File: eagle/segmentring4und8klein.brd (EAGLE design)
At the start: 100 x 150 mm, 12 parts

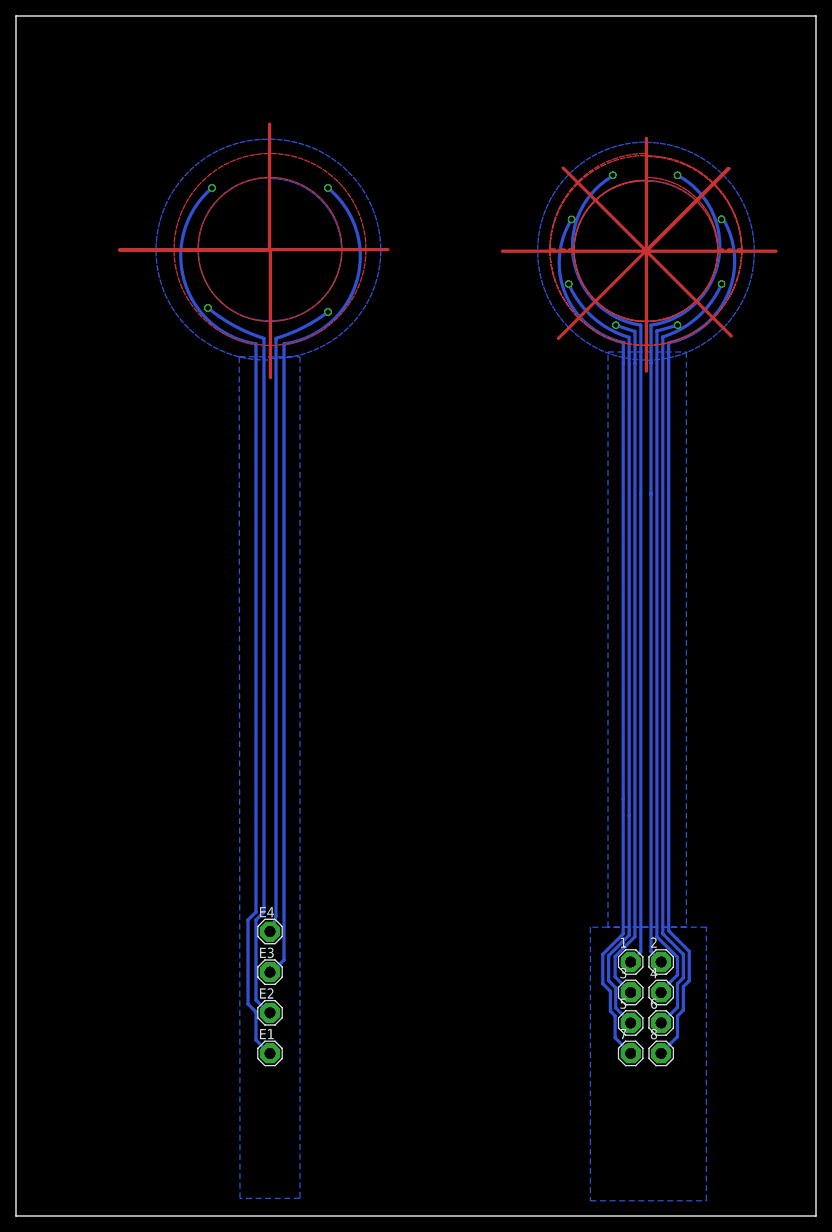
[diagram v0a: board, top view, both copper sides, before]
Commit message: Verbesserung der Boards
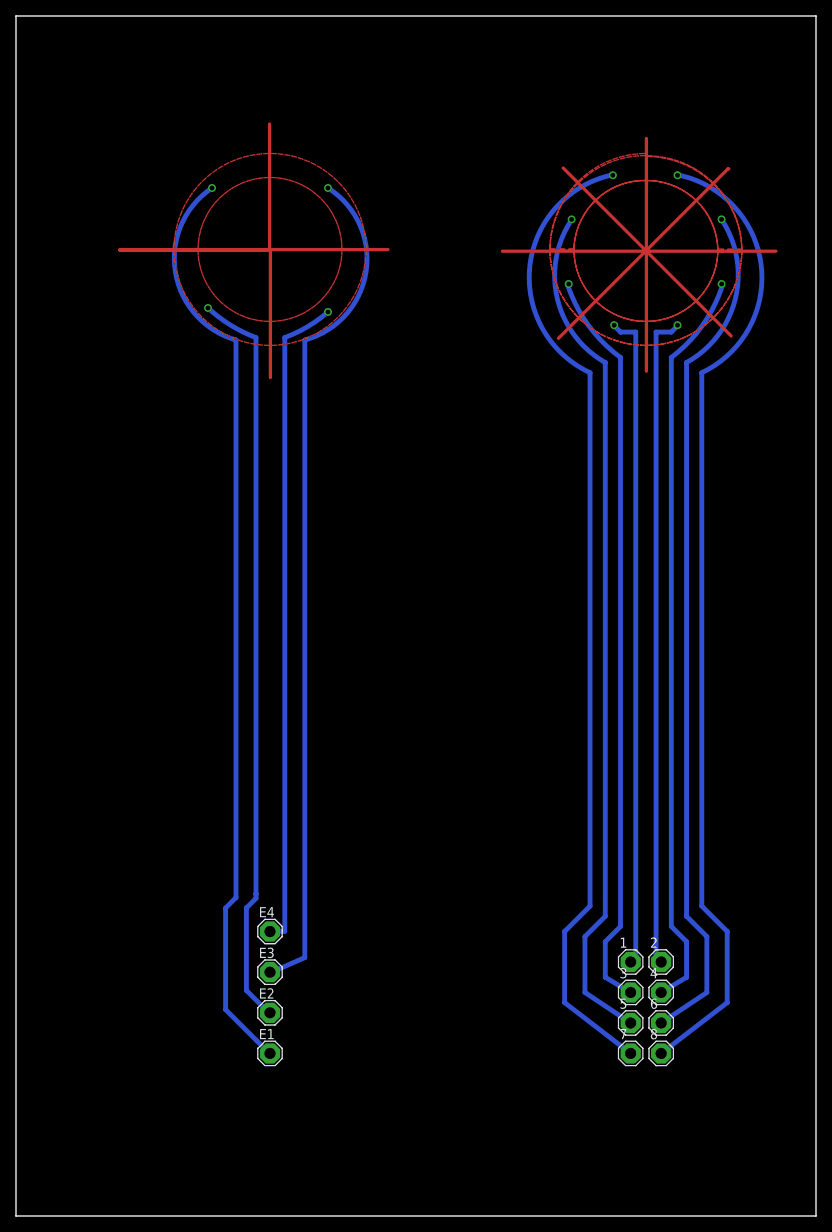
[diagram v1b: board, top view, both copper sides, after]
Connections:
- new net 1: 1.MP
- new net 2: 2.MP
- new net 3: 3.MP
- new net 4: 4.MP
- new net 5: 5.MP
- new net 6: 6.MP
- new net 7: 7.MP
- new net 8: 8.MP
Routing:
- net S$3: track 137.6 -> 93.0 mm
- net S$4: track 0.00 -> 30.1 mm
- net 2: track 99.7 -> 81.8 mm
- net 1: track 99.1 -> 81.8 mm
- net 7: track 108.0 -> 115.4 mm
- net 5: track 97.7 -> 104.9 mm
- net 6: track 98.2 -> 105.0 mm
- net 8: track 108.7 -> 115.4 mm
- net 3: track 86.9 -> 93.0 mm
- net 4: track 87.3 -> 92.9 mm
- net E3: track 99.4 -> 100.9 mm
- net E1: track 110.2 -> 111.0 mm
- net E4: track 81.6 -> 82.3 mm
- removed copper zone on layer 16, net GND
- removed copper zone on layer 16, net N$8
